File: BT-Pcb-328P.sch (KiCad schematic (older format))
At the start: 64 parts, among them J1 USB_B_Micro, J2 FTDI, J3 ICSP, J4 ANT, J5 Si7021, J6 Vin, P1 MYSX_2.6, Q1 FDN338P, Q2 FDN337N, Q3 FDN337N, Q4 FDN338P, Q5 FDN338P, Q6 FDN337N, SW1 1437566-3, SW2 1437566-3, U1 AMS1117-3.3, U2 AS312, U3 ATmega328P-AU, U4 RFM69HW, U5 ME2188C33, U6 ATSHA204A, U7 NRF24L01, U8 NRF24L01

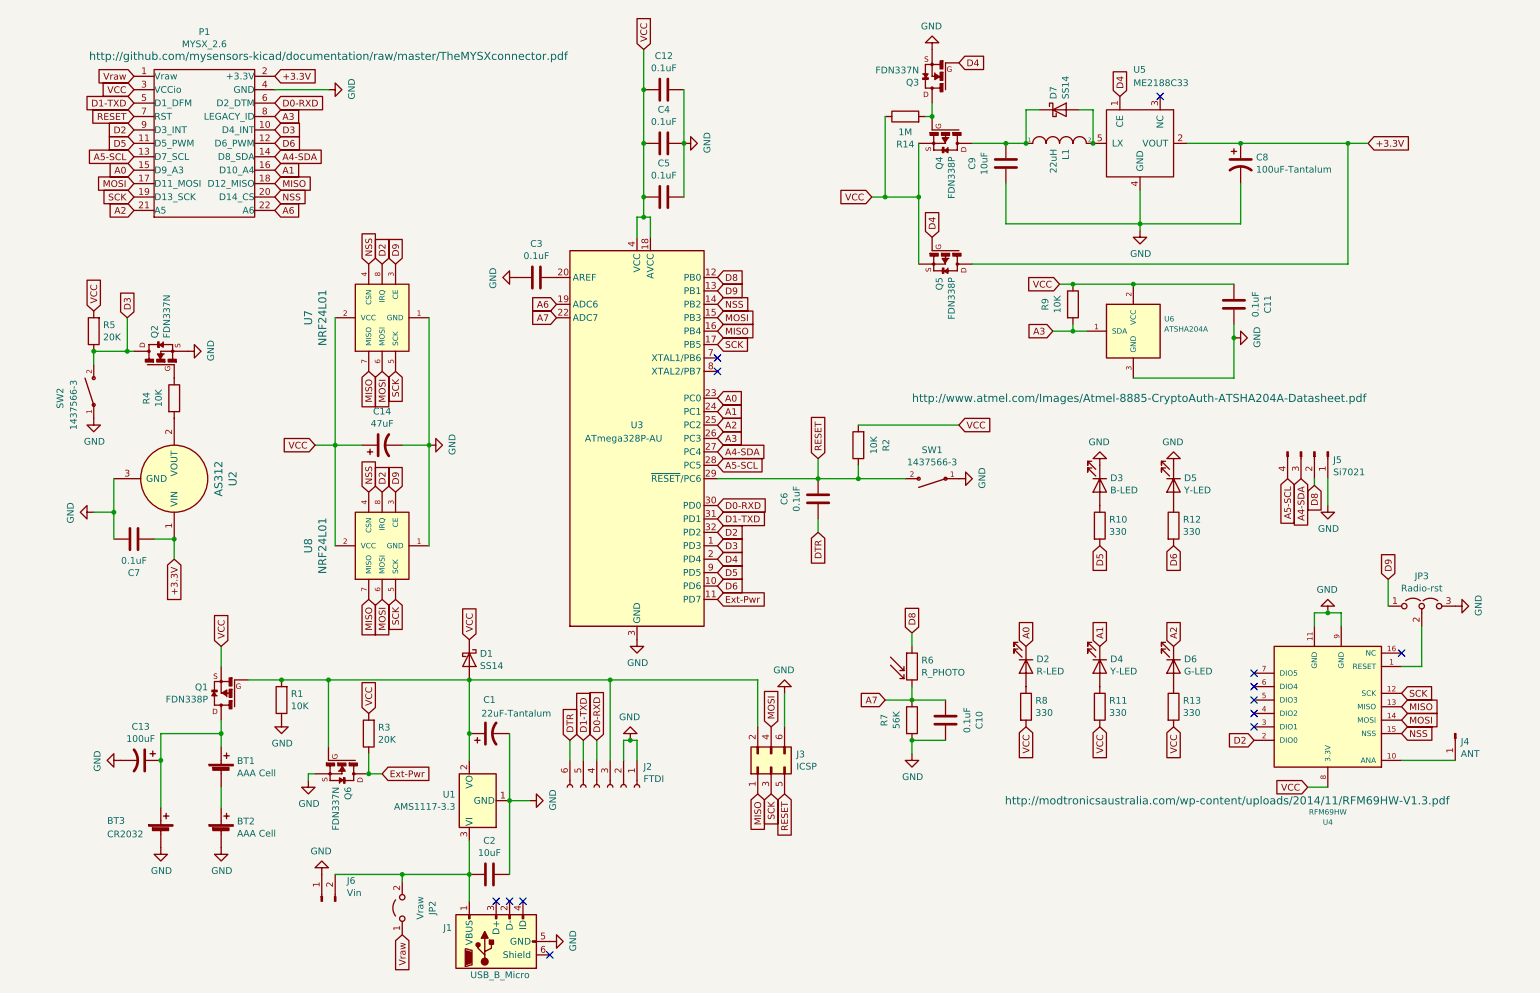
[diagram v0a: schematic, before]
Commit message: board v.2.0
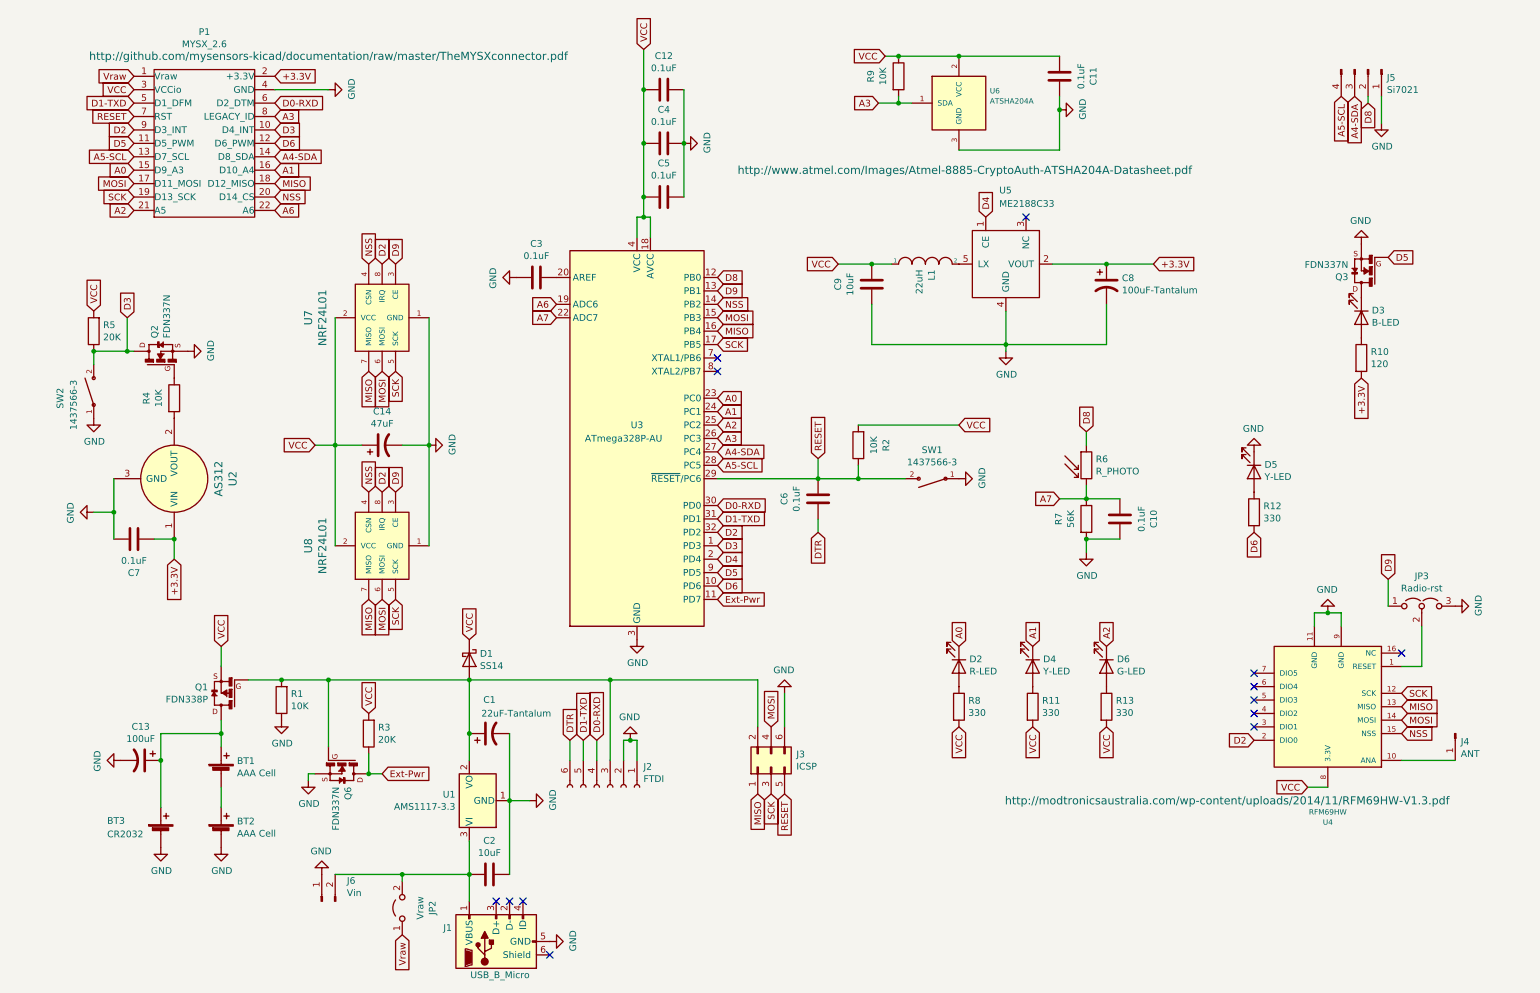
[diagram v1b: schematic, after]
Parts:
- removed D7: SS14, diodes:SS14, symbol Device:D_Schottky
- removed Q4, Q5: FDN338P, FDN338P:SSOT-3, symbol FDN338P:FDN338P
- removed R14: 1M, Resistor_SMD:R_0805_2012Metric, symbol Device:R
- R10: value 330 -> 120
- U2: footprint as312:as312 -> as312:PIR-AS312-3PIN
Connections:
- net +3.3V: now also R10.2
- net D4: no longer Q3.1 (G)
- net D5: now also Q3.1 (G); no longer R10.2
- net GND: no longer D3.1 (K)
- net VCC: now also C9.2, L1.1
- net at Q3.3 (D): now also D3.1 (K)
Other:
- moved on the sheet: C10, C11, C8, C9, D2, D3, D4, D5, D6, J5, L1, R10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
